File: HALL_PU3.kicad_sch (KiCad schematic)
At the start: 30 parts, among them Q15 AO3400A, Q16 AO3401A, Q17 AO3401A, Q2 AO3400A, Q25 AO3400A, Q31 AO3401A, Q32 AO3401A, Q4 AO3401A, Q5 AO3401A

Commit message: PN fixes
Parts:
- D78: LCSC C408389 -> C47546
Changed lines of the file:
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@@
       (effects (font (size 1.27 1.27)) hide)
     )
-    (property "LCSC" "C408389" (at 125.73 162.56 0)
+    (property "LCSC" "C47546" (at 125.73 162.56 0)
       (effects (font (size 1.27 1.27)) hide)
     )
@@
       (effects (font (size 1.27 1.27)) hide)
     )
-    (property "LCSC" "C408389" (at 125.73 64.77 0)
+    (property "LCSC" "C47546" (at 125.73 64.77 0)
       (effects (font (size 1.27 1.27)) hide)
     )
@@
       (effects (font (size 1.27 1.27)) hide)
     )
-    (property "LCSC" "C408389" (at 125.73 114.3 0)
-      (effects (font (size 1.27 1.27)) hide)
-    )
+    (property "LCSC" "C47546" (at 125.73 114.3 0)
+      (effects (font (size 1.27 1.27)) hide)
+    )

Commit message: Rev H*: #140, #142, #144, #145
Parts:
- R21, R23, R34, R36, R75, R77: footprint hellen-one-common:R1206 -> Resistor_SMD:R_1206_3216Metric
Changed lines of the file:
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@@
       (effects (font (size 1.27 1.27)))
     )
-    (property "Footprint" "hellen-one-common:R1206" (at 107.95 113.03 0)
+    (property "Footprint" "Resistor_SMD:R_1206_3216Metric" (at 107.95 113.03 0)
       (effects (font (size 1.27 1.27)) hide)
     )
@@
       (effects (font (size 1.27 1.27)))
     )
-    (property "Footprint" "hellen-one-common:R1206" (at 118.11 161.29 0)
+    (property "Footprint" "Resistor_SMD:R_1206_3216Metric" (at 118.11 161.29 0)
       (effects (font (size 1.27 1.27)) hide)
     )
@@
       (effects (font (size 1.27 1.27)))
     )
-    (property "Footprint" "hellen-one-common:R1206" (at 118.11 63.5 0)
+    (property "Footprint" "Resistor_SMD:R_1206_3216Metric" (at 118.11 63.5 0)
       (effects (font (size 1.27 1.27)) hide)
     )
@@
       (effects (font (size 1.27 1.27)))
     )
-    (property "Footprint" "hellen-one-common:R1206" (at 107.95 63.5 0)
+    (property "Footprint" "Resistor_SMD:R_1206_3216Metric" (at 107.95 63.5 0)
       (effects (font (size 1.27 1.27)) hide)
     )
@@
       (effects (font (size 1.27 1.27)))
     )
-    (property "Footprint" "hellen-one-common:R1206" (at 118.11 113.03 0)
+    (property "Footprint" "Resistor_SMD:R_1206_3216Metric" (at 118.11 113.03 0)
       (effects (font (size 1.27 1.27)) hide)
     )
@@
       (effects (font (size 1.27 1.27)))
     )
-    (property "Footprint" "hellen-one-common:R1206" (at 107.95 161.29 0)
-      (effects (font (size 1.27 1.27)) hide)
-    )
+    (property "Footprint" "Resistor_SMD:R_1206_3216Metric" (at 107.95 161.29 0)
+      (effects (font (size 1.27 1.27)) hide)
+    )

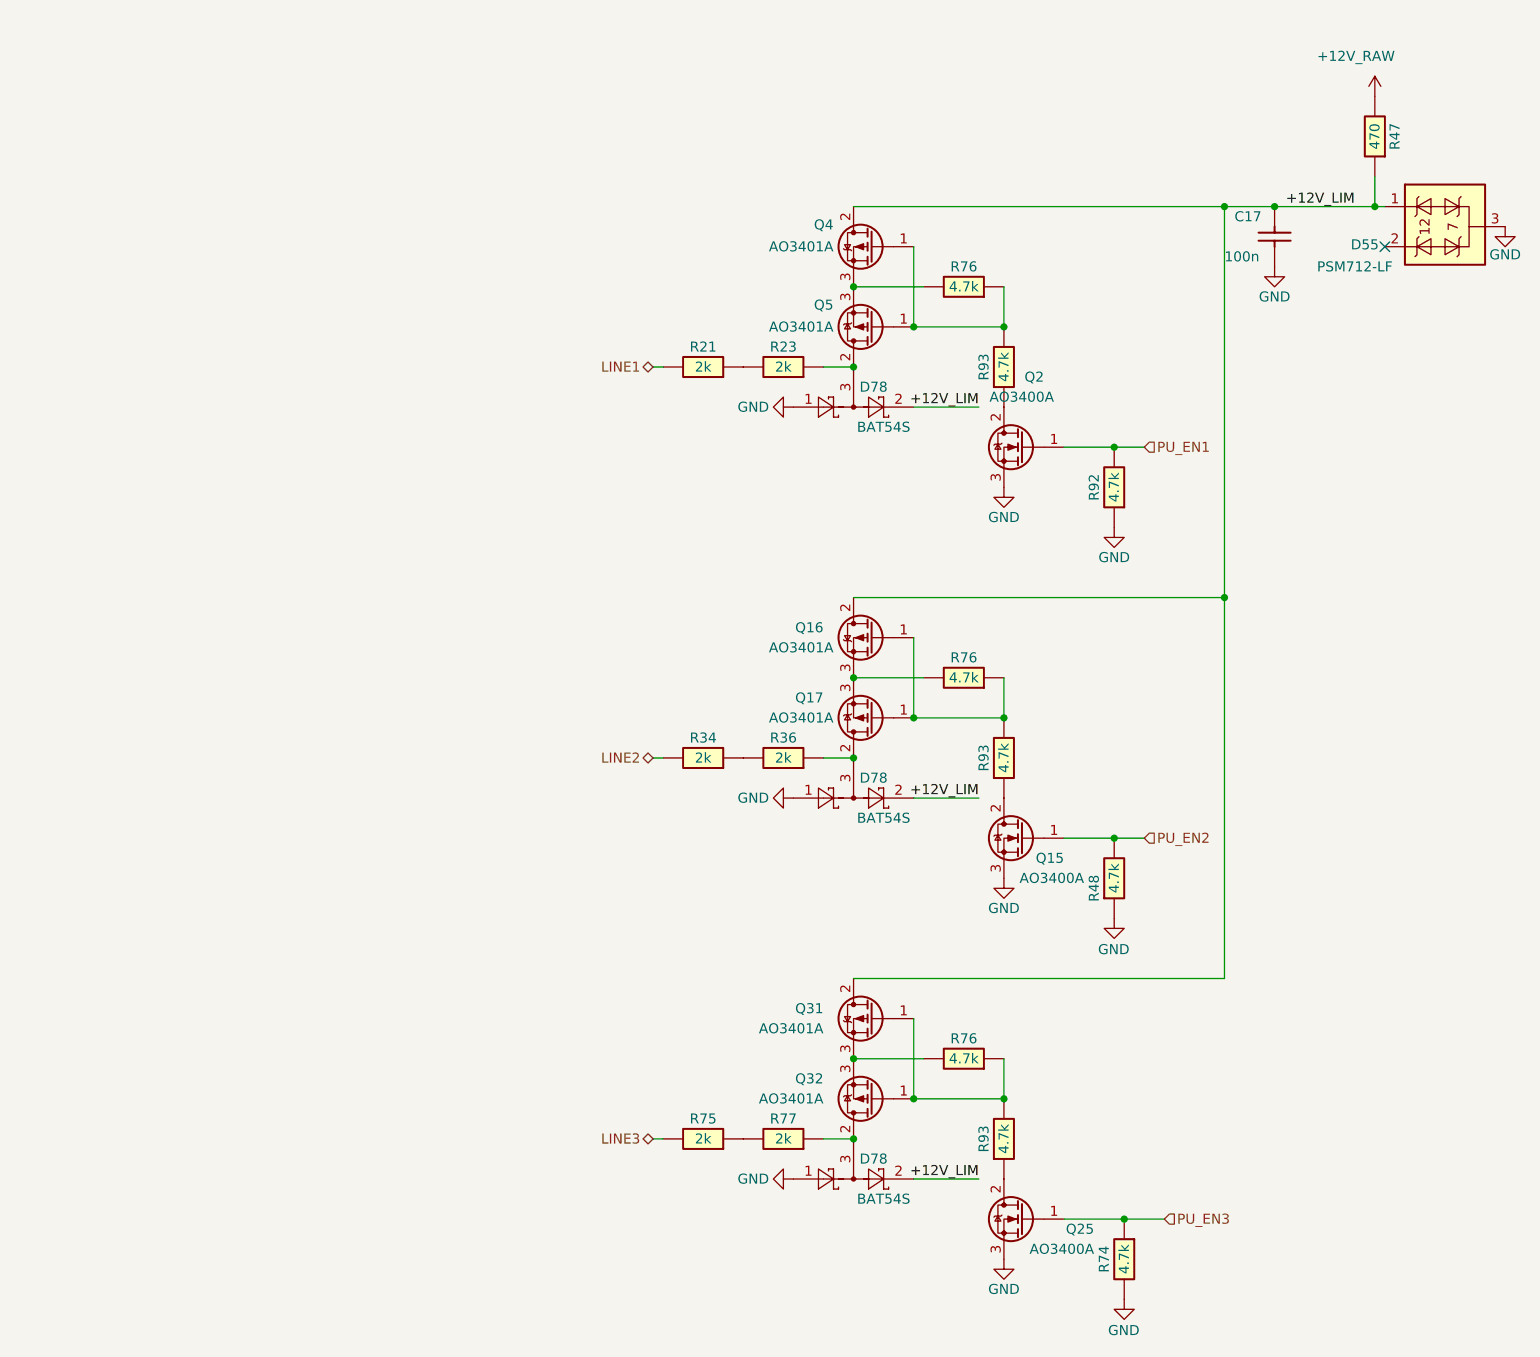
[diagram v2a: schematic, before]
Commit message: Export
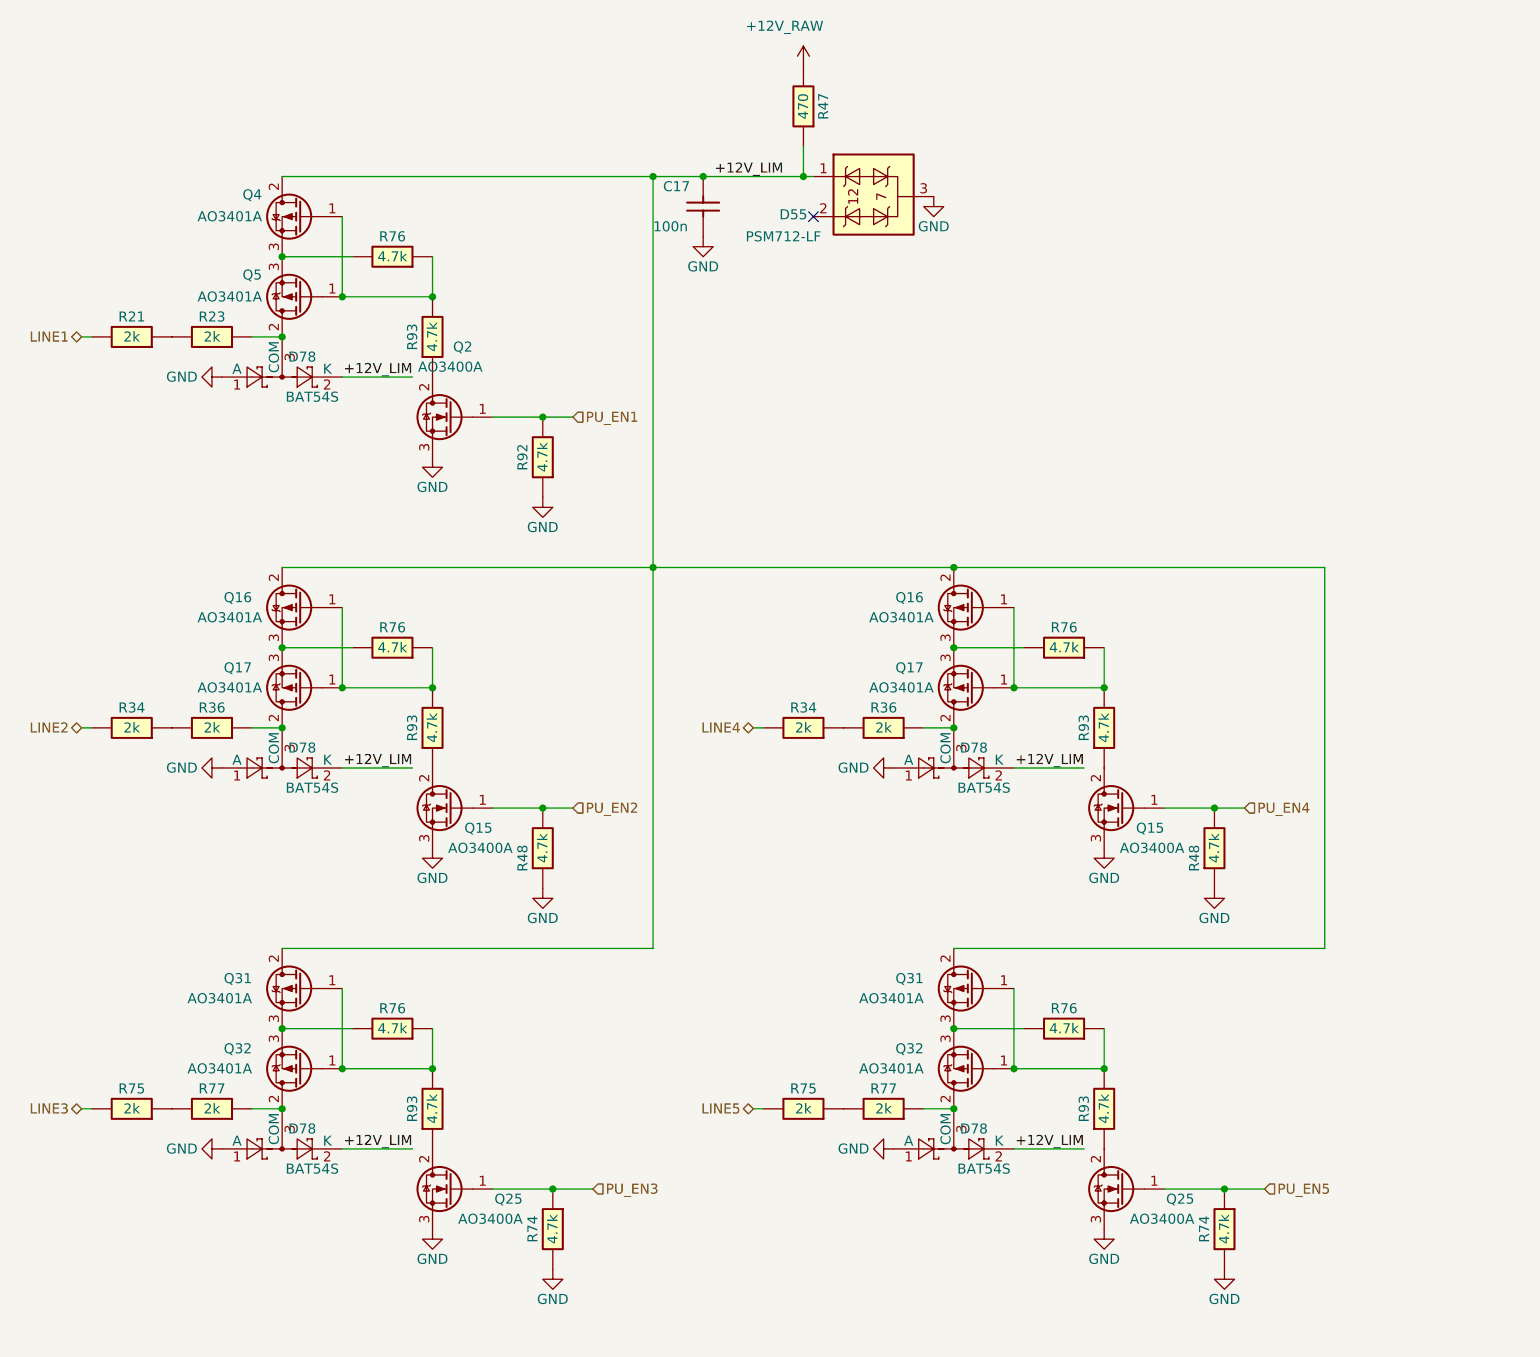
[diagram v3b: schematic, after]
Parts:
- added D78 (x2): BAT54S, Package_TO_SOT_SMD:SOT-23, symbol Diode:BAT54S
- added Q15, Q25: AO3400A, hellen-one-common:SOT-23, symbol hellen-one-common:MOSFET-N
- added Q16, Q17, Q31, Q32: AO3401A, hellen-one-common:SOT-23, symbol hellen-one-common:MOSFET-P
- added R34, R36, R75, R77: 2k, Resistor_SMD:R_1206_3216Metric, symbol hellen-one-common:Res
- added R48, R74, R76 (x2), R93 (x2): 4.7k, hellen-one-common:R0603, symbol hellen-one-common:Res
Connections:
- net +12V_LIM: now also D78.2 (K), D78.2 (K), Q16.2 (D), Q31.2 (D)
- net GND: now also D78.1 (A), D78.1 (A), Q15.3 (S), Q25.3 (S), R48.1, R74.2
- new net: Q31.1 (G), Q32.1 (G), R76.1, R93.2
- new net: D78.3 (COM), Q32.2 (D), R77.1
- new net: Q31.3 (S), Q32.3 (S), R76.2
- new net: D78.3 (COM), Q17.2 (D), R36.1
- new net: R75.1, R77.2
- new net: R34.1, R36.2
- new net: Q16.1 (G), Q17.1 (G), R76.1, R93.2
- new net: Q16.3 (S), Q17.3 (S), R76.2
- new net: Q15.2 (D), R93.1
- new net: Q25.2 (D), R93.1
- new net LINE4: R34.2
- new net LINE5: R75.2
- new net PU_EN4: Q15.1 (G), R48.2
- new net PU_EN5: Q25.1 (G), R74.1
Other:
- moved on the sheet: C17, D55, Q15, Q16, Q17, Q2, Q25, Q31, Q32, Q4, Q5, R21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
